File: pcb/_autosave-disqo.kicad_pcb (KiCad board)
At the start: 4 copper layers, 40 x 38.3 mm, 76 parts, among them IC1 AS5600-ASOT, J1 USB4105-GF-A, J2 Conn_01x02, Q1 DMN2004VK-7, Q2 DMP2004VK-7, Q3 DMN2004VK-7, SW1 top-switch, SW2 top-switch, SW3 side-switch, SW4 side-switch, SW5 side-switch, U1 MCP73831-2-OT, U2 CP2102N-Axx-xQFN24, U3 ESP32-PICO-V3, U4 AP7354-33W5-7, U5 GC9A01, Y1 32.768kHz 6pF

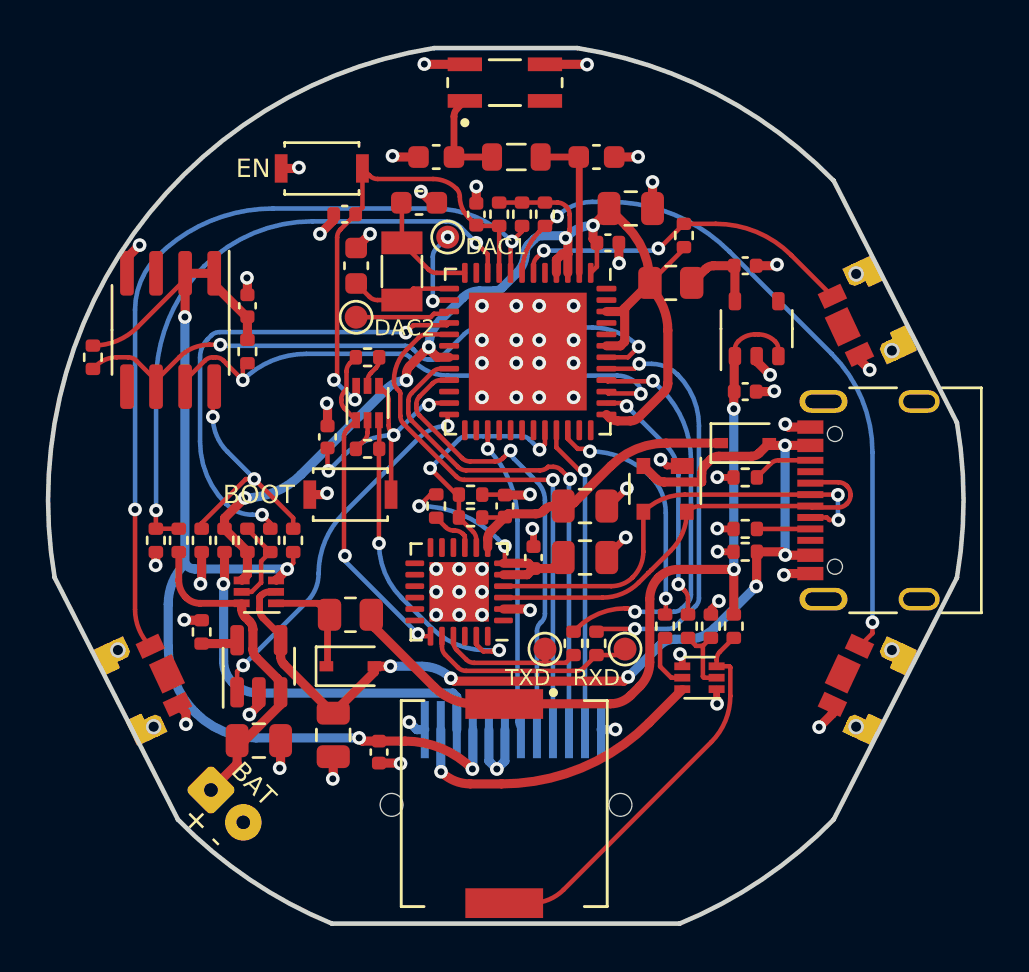
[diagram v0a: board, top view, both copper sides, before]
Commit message: pcb changes
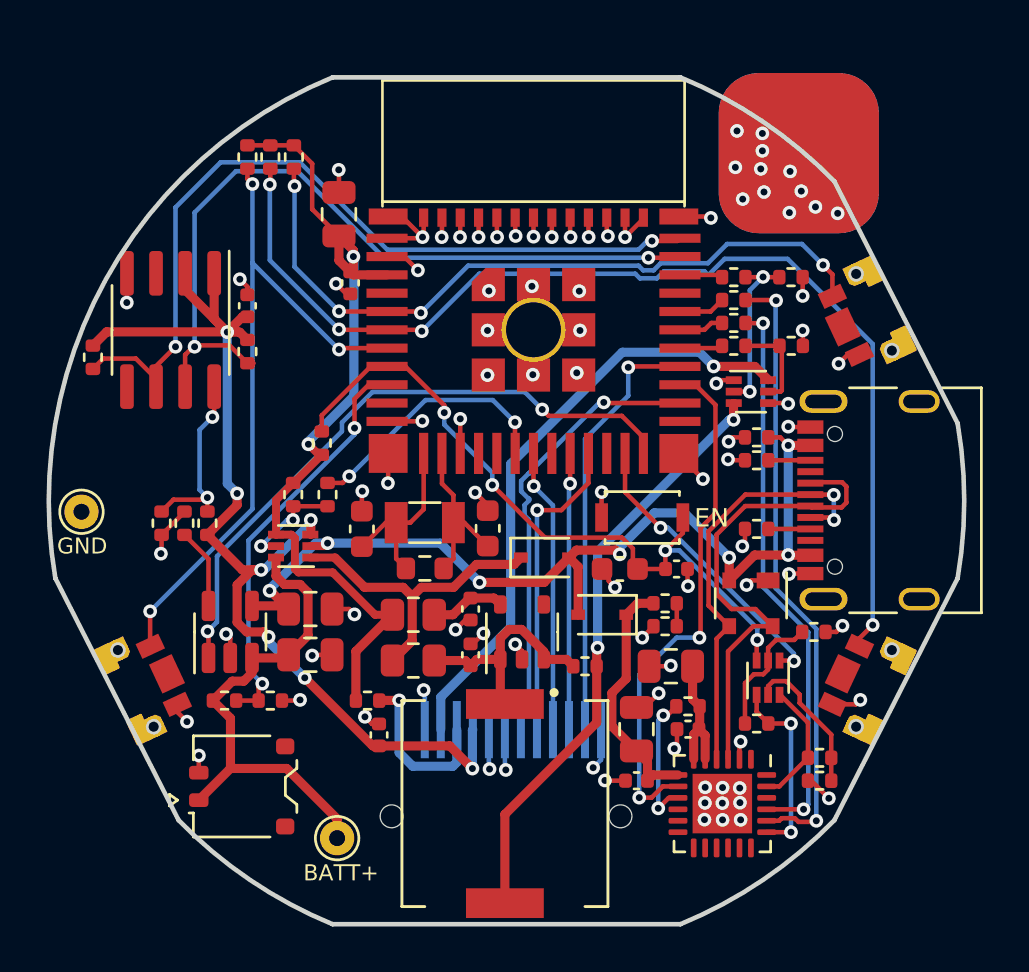
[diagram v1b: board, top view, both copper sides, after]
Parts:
- removed C12: 0.1uF, Capacitor_SMD:C_0402_1005Metric
- removed C18, C19: TBD, Capacitor_SMD:C_0603_1608Metric
- removed E1: 2450AT42E0100E, 2450AT42E0100:XDCR_2450AT42E0100E
- removed L1: 0R, Inductor_SMD:L_0805_2012Metric
- removed SW2: top-switch, KXT-311:KXT 311 LHS
- removed TP6: TXD, testpoint:TestPoint_Pad_D1.0mm
- removed TP7: RXD, testpoint:TestPoint_Pad_D1.0mm
- added R14: 6.8M, Resistor_SMD:R_0603_1608Metric, F.Cu at (96.5, 103.0)
- added R32: 100k, Resistor_SMD:R_0402_1005Metric, F.Cu at (113.8, 112.2)
- added R33: 100k, Resistor_SMD:R_0402_1005Metric, F.Cu at (113.5, 105.8)
- added R34: 100k, Resistor_SMD:R_0402_1005Metric, F.Cu at (112.5, 93.2)
- added TP3: GND, tab:tab, F.Cu at (112.8, 84.8)
- added TP4: GND, tab:tab, B.Cu at (112.8, 84.8)
- C15: value 0.1uF -> 1uF; footprint Capacitor_SMD:C_0402_1005Metric -> Capacitor_SMD:C_0603_1608Metric
- C16: value 10uF -> 22uF
- J2: footprint battery-connector:Battery Connector -> Connector_JST:JST_ACH_BM02B-ACHSS-GAN-ETF_1x02-1MP_P1.20mm_Vertical
- TP1: value DAC1 -> BATT+; footprint testpoint:TestPoint_Pad_D1.0mm -> TestPoint:TestPoint_THTPad_D1.5mm_Drill0.7mm
- TP2: value DAC2 -> GND; footprint testpoint:TestPoint_Pad_D1.0mm -> TestPoint:TestPoint_THTPad_D1.5mm_Drill0.7mm
- U3: value ESP32-PICO-V3 -> ESP32-PICO-MINI-02; footprint Package_DFN_QFN:QFN-48-1EP_7x7mm_P0.5mm_EP5.15x5.15mm -> Espressif:ESP32-PICO-MINI-02_Hand-Soldering
- moved TP1 26.7 mm to (92.7, 114.8)
- moved R10 23.9 mm to (113.8, 111.2), turned to 180 degrees
- moved R11 23.3 mm to (111.0, 109.8), turned to 0 degrees
- moved C11 21.2 mm to (107.5, 103.0), turned to 0 degrees
- moved Q1 21.2 mm to (111.5, 107.8)
- moved SW1 20.7 mm to (106.0, 100.8)
- moved C3 19.2 mm to (98.5, 104.8), turned to -90 degrees
- moved R12 18.4 mm to (96.0, 105.0)
- moved R29 17.4 mm to (90.8, 85.0), turned to 90 degrees
- moved U4 16.8 mm to (100.8, 105.8)
- moved C15 16.7 mm to (105.0, 103.0), turned to 180 degrees
- moved C2 16.6 mm to (98.5, 106.8), turned to 90 degrees
- moved R9 16.2 mm to (110.0, 91.2), turned to 0 degrees
- moved R8 15.7 mm to (110.0, 92.2), turned to 0 degrees
- moved R20 15.6 mm to (112.5, 90.2), turned to 0 degrees
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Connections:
- TP1 pad 1: /DAC1 -> +BATT
- TP2 pad 1: /DAC2 -> GND
- U3 pad 1: +3V3 -> GND
- U3 pad 10: /BATT_ADC -> unconnected-(U3-Pad10)
- U3 pad 11: unconnected-(U3-Pad11) -> GND
- U3 pad 14: /DAC1 -> GND
- U3 pad 15: /DAC2 -> /DAC1
- U3 pad 16: /ENABLE -> /DAC2
- U3 pad 17: /SCLK -> /ENABLE
- U3 pad 18: unconnected-(U3-Pad18) -> /SCLK
- U3 pad 19: +3V3 -> unconnected-(U3-Pad19)
- U3 pad 2: /LNA_IN -> GND
- U3 pad 26: unconnected-(U3-Pad26) -> /LCD_DC
- U3 pad 27: /LCD_DC -> /CONNECTED
- U3 pad 28: unconnected-(U3-Pad28) -> /LCD_RESET
- U3 pad 29: unconnected-(U3-Pad29) -> /PIEZO
- U3 pad 30: unconnected-(U3-Pad30) -> /RXD0
- U3 pad 31: unconnected-(U3-Pad31) -> /TXD0
- U3 pad 32: /CONNECTED -> unconnected-(U3-Pad32)
- U3 pad 33: /LCD_RESET -> /BACKLIGHT
- U3 pad 34: /PIEZO -> /SCL
- U3 pad 35: unconnected-(U3-Pad35) -> /SDA
- U3 pad 36: unconnected-(U3-Pad36) -> GND
- U3 pad 4: +3V3 -> unconnected-(U3-Pad4)
- U3 pad 5: unconnected-(U3-Pad5) -> /B1
- U3 pad 6: /B1 -> /B2
- U3 pad 7: /B2 -> /B3
- U3 pad 8: /B3 -> /EN
- U3 pad 9: /EN -> /BATT_ADC
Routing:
- net VCC: track 36.5 -> 10.3 mm, vias 2 -> 0
- net GND: track 48.4 -> 68.8 mm, vias 70 -> 91
- net /TXD: track 6.73 -> 24.5 mm, vias 0 -> 2
- net /RXD: track 9.34 -> 27.1 mm, vias 0 -> 2
- net +3V3: track 55.7 -> 38.0 mm, vias 5 -> 2
- net /B2: track 31.1 -> 48.2 mm, vias 2 -> 4
- net /TXD0: track 18.5 -> 2.05 mm, vias 2 -> 0
- net /B1: track 15.3 -> 31.6 mm, vias 2 -> 4
- net /RXD0: track 17.7 -> 1.96 mm, vias 2 -> 0
- net /CONNECTED: track 10.8 -> 23.9 mm
- net /LEDK: track 13.8 -> 26.6 mm
- net /STAT: track 16.1 -> 28.0 mm
- net /SCLK: track 24.0 -> 12.4 mm
- net /MOSI: track 22.3 -> 12.1 mm
- net /EN: track 20.9 -> 31.1 mm, vias 2 -> 4
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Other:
- board size 40 x 38.3 mm -> 40 x 37 mm
- board text added: "TODO: exposed gnd and other areas for crocodile clips in the unused space"
- board text removed: "+ -"
- board text removed: "BAT"
- board text removed: "MCP73831 max 1.45mm thick"
- board text removed: "Piezo is 1.9mm thick max"
- board text removed: "current design leaves 1.75 max with 0.75mm thinnest cover thickness. could make that 0.6mm thin and have 1.9mm piezo?"
